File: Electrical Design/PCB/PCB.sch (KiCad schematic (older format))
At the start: 57 parts, among them J1 Conn_02x03_Odd_Even, J2 10118193-0001LF, M1 Camera_Servo, M2 Release_Servo, Q1 LED_MOS, Q2 CAMERA_MOS, Q3 RELEASE_MOS, Q4 BUZZER_MOS, U1 ADP3338AKCZ-5-R7, U2 BNO080, U3 ADP3338AKCZ-3.3-R7, U4 PCF8523T_1_118, U5 MS560702BA03-50, U6 SS495A, U7 Adafruit_746, U8 Openlog, U9 ATxmega128A4U-AU

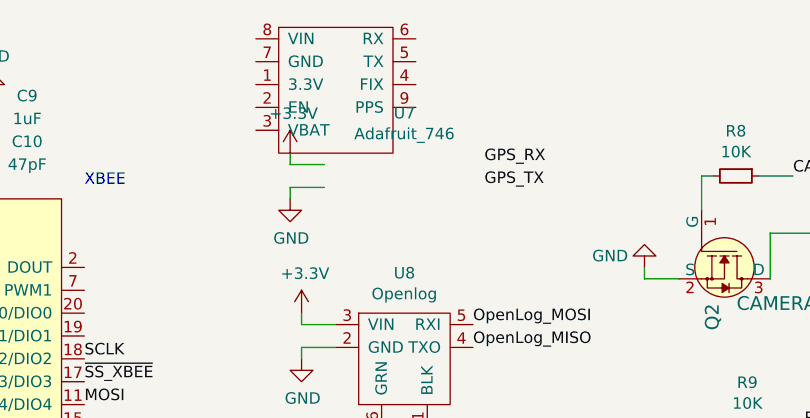
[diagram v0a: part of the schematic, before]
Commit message: Netlist
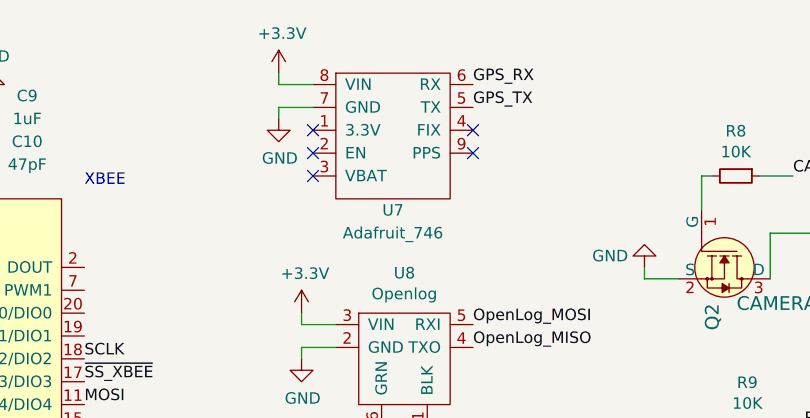
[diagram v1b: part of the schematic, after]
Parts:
- C13, C15: footprint (none) -> Capacitor_THT:CP_Radial_D10.0mm_P5.00mm
- C2, C3, C5: footprint (none) -> Capacitor_THT:CP_Radial_D5.0mm_P2.00mm
- U7: footprint (none) -> Connectors:1X09
- U8: footprint (none) -> Connectors:1X06
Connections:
- net +3V3: now also U7.8 (VIN)
- net GND: now also U7.7 (GND)
- net GPS_RX: now also U7.6 (RX)
- net GPS_TX: now also U7.5 (TX)
- no-connect marks 7 -> 12
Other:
- moved on the sheet: U7
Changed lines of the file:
@@
 F 0 "C13" V 7050 5550 50  0000 C CNN
 F 1 "10uF" V 7150 5550 50  0000 C CNN
-F 2 "" H 7100 5850 50  0001 C CNN
+F 2 "Capacitor_THT:CP_Radial_D10.0mm_P5.00mm" H 7100 5850 50  0001 C CNN
 F 3 "~" H 7100 5850 50  0001 C CNN
 	1    7100 5850
@@
 F 0 "C15" V 7550 5300 50  0000 C CNN
 F 1 "10uF" V 7450 5300 50  0000 C CNN
-F 2 "" H 7500 5550 50  0001 C CNN
+F 2 "Capacitor_THT:CP_Radial_D10.0mm_P5.00mm" H 7500 5550 50  0001 C CNN
 F 3 "~" H 7500 5550 50  0001 C CNN
 	1    7500 5550
@@
 F 0 "C2" H 1350 1200 50  0000 L CNN
 F 1 "0.1uF" H 1300 1100 50  0000 L CNN
-F 2 "" H 1400 900 50  0001 C CNN
+F 2 "Capacitor_THT:CP_Radial_D5.0mm_P2.00mm" H 1400 900 50  0001 C CNN
 F 3 "~" H 1400 900 50  0001 C CNN
 	1    1400 900
@@
 F 0 "C3" H 1600 1200 50  0000 L CNN
 F 1 "0.1uF" H 1550 1100 50  0000 L CNN
-F 2 "" H 1650 900 50  0001 C CNN
+F 2 "Capacitor_THT:CP_Radial_D5.0mm_P2.00mm" H 1650 900 50  0001 C CNN
 F 3 "~" H 1650 900 50  0001 C CNN
 	1    1650 900
@@
 F 0 "C5" H 2791 2996 50  0000 L CNN
 F 1 "0.1uF" H 2791 2905 50  0000 L CNN
-F 2 "" H 2700 2950 50  0001 C CNN
+F 2 "Capacitor_THT:CP_Radial_D5.0mm_P2.00mm" H 2700 2950 50  0001 C CNN
 F 3 "~" H 2700 2950 50  0001 C CNN
 	1    2700 2950
@@
 L Skyfire_Custom_Components:Adafruit_746 U7
 U 1 1 5C5FC17D
-P 7200 1150
-F 0 "U7" H 6900 1475 50  0000 C CNN
-F 1 "Adafruit_746" H 6900 1384 50  0000 C CNN
-F 2 "" H 7200 1150 50  0001 C CNN
-F 3 "" H 7200 1150 50  0001 C CNN
-	1    7200 1150
-	1    0    0    -1
-$EndComp
-Text Label 7250 1150 0    50   ~ 0
+P 7450 1350
+F 0 "U7" H 6850 1450 50  0000 C CNN
+F 1 "Adafruit_746" H 6850 1350 50  0000 C CNN
+F 2 "Connectors:1X09" H 7450 1350 50  0001 C CNN
+F 3 "" H 7450 1350 50  0001 C CNN
+	1    7450 1350
+	1    0    0    -1
+$EndComp
+Text Label 7200 800  0    50   ~ 0
 GPS_TX
-Text Label 7250 1050 0    50   ~ 0
+Text Label 7200 700  0    50   ~ 0
 GPS_RX
 Text Label 8950 5150 2    50   ~ 0
@@
 L power:+3.3V #PWR033
 U 1 1 5C6096AA
-P 6400 1000
-F 0 "#PWR033" H 6400 850 50  0001 C CNN
-F 1 "+3.3V" H 6415 1173 50  0000 C CNN
-F 2 "" H 6400 1000 50  0001 C CNN
-F 3 "" H 6400 1000 50  0001 C CNN
-	1    6400 1000
+P 6350 650
+F 0 "#PWR033" H 6350 500 50  0001 C CNN
+F 1 "+3.3V" H 6365 823 50  0000 C CNN
+F 2 "" H 6350 650 50  0001 C CNN
+F 3 "" H 6350 650 50  0001 C CNN
+	1    6350 650
 	1    0    0    -1
 $EndComp
@@
 L power:GND #PWR034
 U 1 1 5C609986
-P 6400 1200
-F 0 "#PWR034" H 6400 950 50  0001 C CNN
-F 1 "GND" H 6405 1027 50  0000 C CNN
-F 2 "" H 6400 1200 50  0001 C CNN
-F 3 "" H 6400 1200 50  0001 C CNN
-	1    6400 1200
-	1    0    0    -1
-$EndComp
-Wire Wire Line
-	6400 1000 6400 1050
-Wire Wire Line
-	6400 1050 6550 1050
-Wire Wire Line
-	6400 1200 6400 1150
-Wire Wire Line
-	6400 1150 6550 1150
+P 6350 850
+F 0 "#PWR034" H 6350 600 50  0001 C CNN
+F 1 "GND" H 6355 677 50  0000 C CNN
+F 2 "" H 6350 850 50  0001 C CNN
+F 3 "" H 6350 850 50  0001 C CNN
+	1    6350 850
+	1    0    0    -1
+$EndComp
+Wire Wire Line
+	6350 650  6350 700
+Wire Wire Line
+	6350 700  6500 700
+Wire Wire Line
+	6350 850  6350 800
+Wire Wire Line
+	6350 800  6500 800
 $Comp
 L Skyfire_Custom_Components:Openlog U8
@@
 F 0 "U8" H 6900 2475 50  0000 C CNN
 F 1 "Openlog" H 6900 2384 50  0000 C CNN
-F 2 "" H 7300 2000 50  0001 C CNN
+F 2 "Connectors:1X06" H 7300 2000 50  0001 C CNN
 F 3 "" H 7300 2000 50  0001 C CNN
 	1    7300 2000
@@
 Text Label 10350 3550 0    50   ~ 0
 BUZZER_MOS
+NoConn ~ 7200 900
+NoConn ~ 7200 1000
+NoConn ~ 6500 900
+NoConn ~ 6500 1000
+NoConn ~ 6500 1100
 $EndSCHEMATC
